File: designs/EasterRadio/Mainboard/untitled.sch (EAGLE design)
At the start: 50 parts, among them IC1 74HC595D, IC2 74HC595D, IC3 74HC595D, IC4 Analog Digital

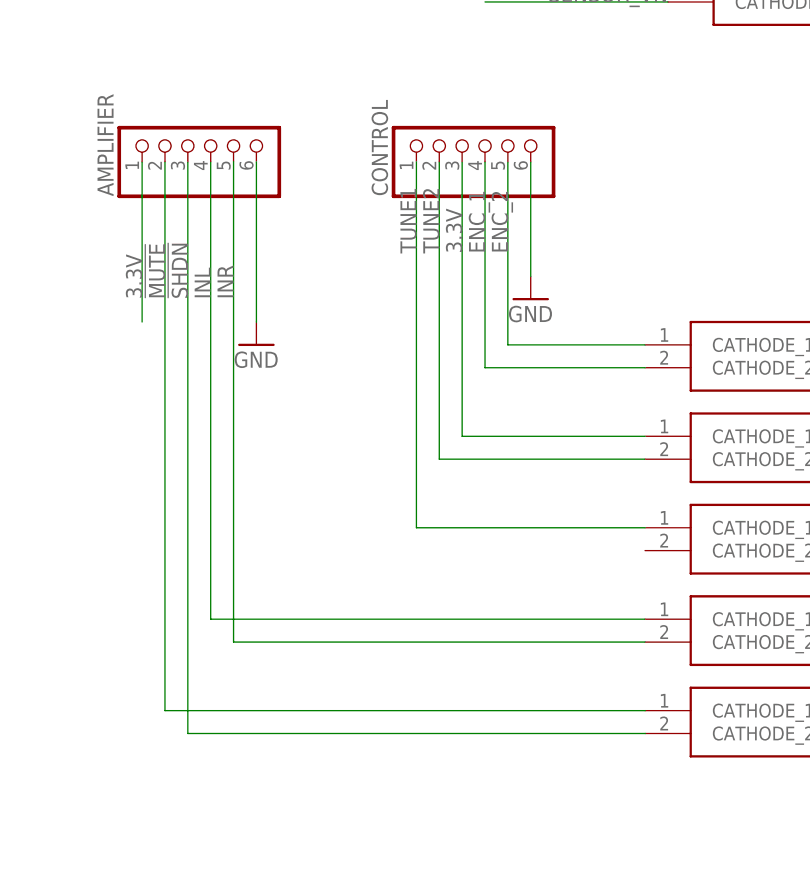
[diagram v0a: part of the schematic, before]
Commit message: final changes on mainboard
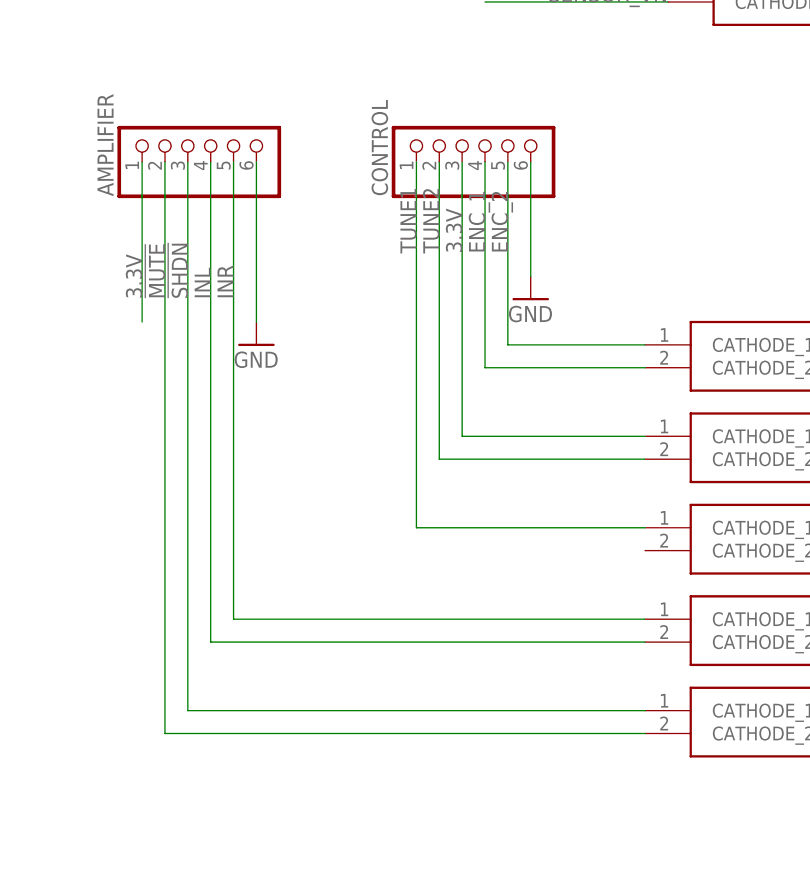
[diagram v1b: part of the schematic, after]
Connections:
- net !MUTE: now also D15.CATHODE_2; no longer D15.CATHODE_1
- net !SHDN: now also D15.CATHODE_1; no longer D15.CATHODE_2
- net INL: now also D14.CATHODE_2; no longer D14.CATHODE_1
- net INR: now also D14.CATHODE_1; no longer D14.CATHODE_2
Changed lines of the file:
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@@
 <pinref part="AMPLIFIER" gate="A" pin="5"/>
 <label x="248.92" y="68.58" size="1.778" layer="95" rot="R90"/>
-<wire x1="248.92" y1="83.82" x2="248.92" y2="30.48" width="0.1524" layer="91"/>
-<pinref part="D14" gate="G$1" pin="CATHODE_2"/>
-<wire x1="248.92" y1="30.48" x2="294.64" y2="30.48" width="0.1524" layer="91"/>
+<wire x1="248.92" y1="83.82" x2="248.92" y2="33.02" width="0.1524" layer="91"/>
+<pinref part="D14" gate="G$1" pin="CATHODE_1"/>
+<wire x1="294.64" y1="33.02" x2="248.92" y2="33.02" width="0.1524" layer="91"/>
 </segment>
 <segment>
@@
 <pinref part="AMPLIFIER" gate="A" pin="4"/>
 <label x="246.38" y="68.58" size="1.778" layer="95" rot="R90"/>
-<wire x1="246.38" y1="83.82" x2="246.38" y2="33.02" width="0.1524" layer="91"/>
-<pinref part="D14" gate="G$1" pin="CATHODE_1"/>
-<wire x1="246.38" y1="33.02" x2="294.64" y2="33.02" width="0.1524" layer="91"/>
+<wire x1="246.38" y1="83.82" x2="246.38" y2="30.48" width="0.1524" layer="91"/>
+<pinref part="D14" gate="G$1" pin="CATHODE_2"/>
+<wire x1="294.64" y1="30.48" x2="246.38" y2="30.48" width="0.1524" layer="91"/>
 </segment>
 <segment>
@@
 <pinref part="AMPLIFIER" gate="A" pin="2"/>
 <label x="241.3" y="68.58" size="1.778" layer="95" rot="R90"/>
-<wire x1="241.3" y1="83.82" x2="241.3" y2="22.86" width="0.1524" layer="91"/>
-<pinref part="D15" gate="G$1" pin="CATHODE_1"/>
-<wire x1="294.64" y1="22.86" x2="241.3" y2="22.86" width="0.1524" layer="91"/>
+<wire x1="241.3" y1="83.82" x2="241.3" y2="20.32" width="0.1524" layer="91"/>
+<pinref part="D15" gate="G$1" pin="CATHODE_2"/>
+<wire x1="294.64" y1="20.32" x2="241.3" y2="20.32" width="0.1524" layer="91"/>
 </segment>
 </net>
@@
 <pinref part="AMPLIFIER" gate="A" pin="3"/>
 <label x="243.84" y="68.58" size="1.778" layer="95" rot="R90"/>
-<wire x1="243.84" y1="83.82" x2="243.84" y2="20.32" width="0.1524" layer="91"/>
-<pinref part="D15" gate="G$1" pin="CATHODE_2"/>
-<wire x1="243.84" y1="20.32" x2="294.64" y2="20.32" width="0.1524" layer="91"/>
+<wire x1="243.84" y1="83.82" x2="243.84" y2="22.86" width="0.1524" layer="91"/>
+<pinref part="D15" gate="G$1" pin="CATHODE_1"/>
+<wire x1="294.64" y1="22.86" x2="243.84" y2="22.86" width="0.1524" layer="91"/>
 </segment>
 </net>
